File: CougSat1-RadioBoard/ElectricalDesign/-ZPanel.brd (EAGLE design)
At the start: 96 x 96 mm, 50 parts, among them J1 High Gain Antenna, J2 Deployables, J3 High Gain +, J4 ADCS, J5 Flap +X, J6 Flap -X, J7 Flap +Y, J8 Flap -Y, U1 AD7291, U2 AD8542, U3 AD8515

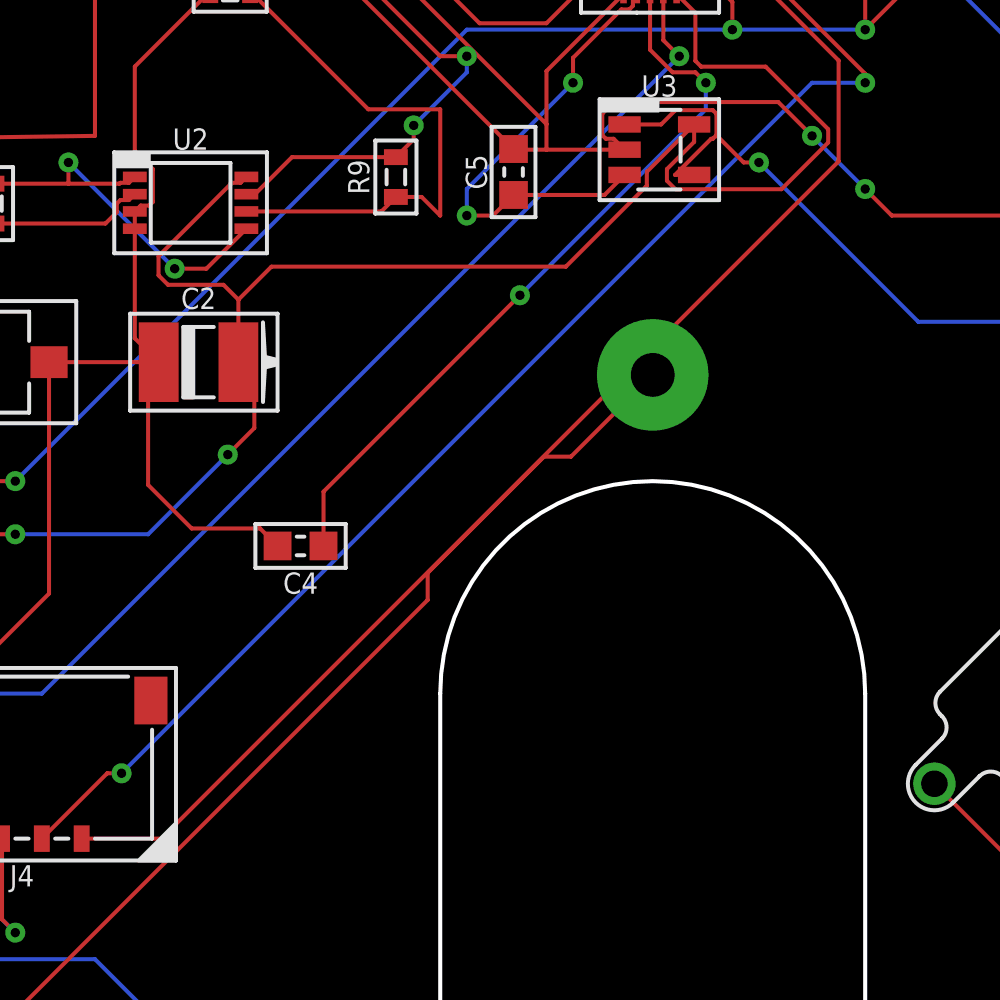
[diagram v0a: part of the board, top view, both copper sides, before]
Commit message: Layout 1.0.0
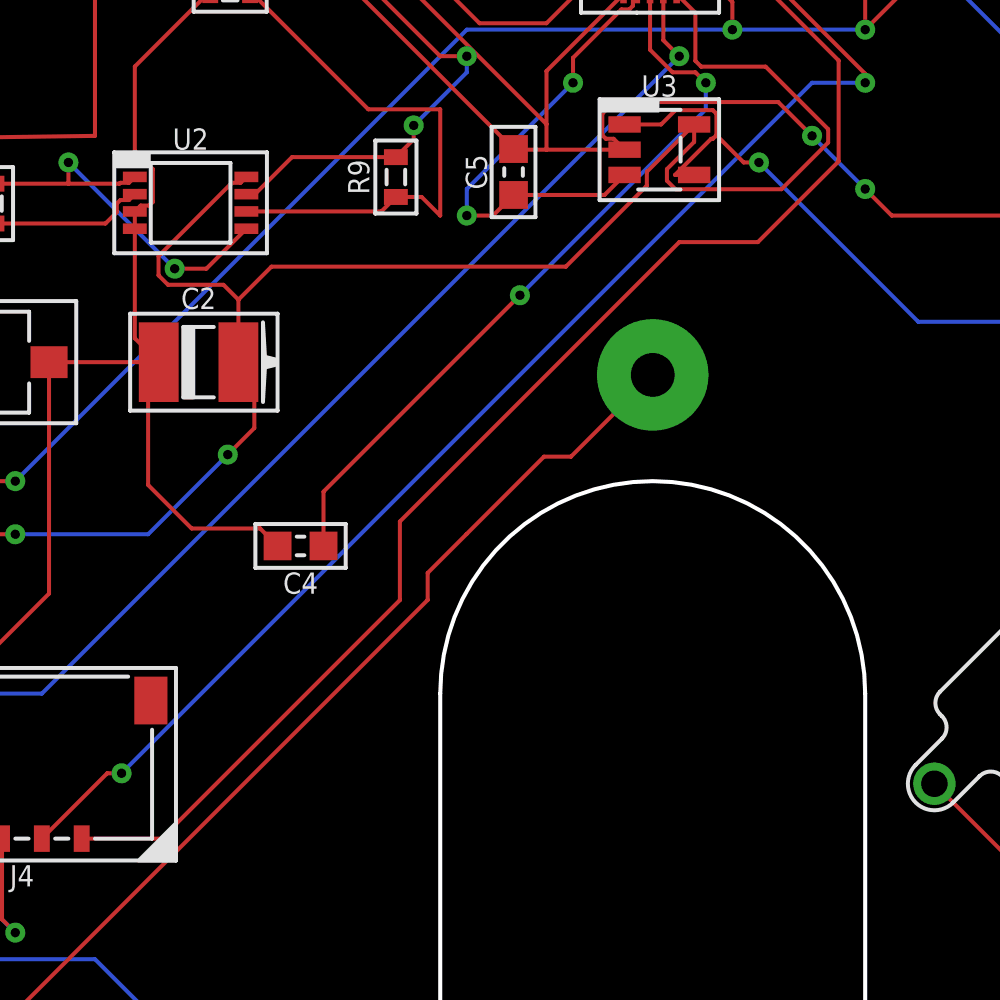
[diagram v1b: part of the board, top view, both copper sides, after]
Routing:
- net I2C_SDA_ADCS: track 50.1 -> 51.8 mm
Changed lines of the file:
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@@
 <contactref element="U1" pad="14"/>
 <contactref element="J4" pad="1"/>
-<wire x1="55" y1="82.04" x2="29.5" y2="56.54" width="0.1524" layer="1"/>
+<wire x1="29.5" y1="56.54" x2="38.48" y2="65.52" width="0.1524" layer="1"/>
 <wire x1="26.5" y1="56.54" x2="29.5" y2="56.54" width="0.1524" layer="1"/>
 <wire x1="50.2446875" y1="90.5936" x2="49.9464" y2="90.5936" width="0.1524" layer="1"/>
@@
 <wire x1="55" y1="85.8382875" x2="50.2446875" y2="90.5936" width="0.1524" layer="1"/>
 <wire x1="55" y1="82.04" x2="55" y2="85.8382875" width="0.1524" layer="1"/>
+<wire x1="38.48" y1="65.52" x2="38.48" y2="68.48" width="0.1524" layer="1"/>
+<wire x1="38.48" y1="68.48" x2="49" y2="79" width="0.1524" layer="1"/>
+<wire x1="49" y1="79" x2="51.96" y2="79" width="0.1524" layer="1"/>
+<wire x1="51.96" y1="79" x2="55" y2="82.04" width="0.1524" layer="1"/>
 </signal>
 <signal name="I2C_SCL_ADCS">
@@
 <wire x1="44.922309375" y1="70.922309375" x2="48" y2="74" width="0.1524" layer="1"/>
 <wire x1="39.526871875" y1="65.526871875" x2="39.526871875" y2="66.542471875" width="0.1524" layer="1"/>
-<wire x1="39.526871875" y1="66.542471875" x2="43.906709375" y2="70.922309375" width="0.1524" layer="1"/>
+<wire x1="39.526871875" y1="66.542471875" x2="40.9922" y2="68.0078" width="0.1524" layer="1"/>
+<wire x1="40.9922" y1="68.0078" x2="43.906709375" y2="70.922309375" width="0.1524" layer="1"/>
 <wire x1="43.906709375" y1="70.922309375" x2="44.922309375" y2="70.922309375" width="0.1524" layer="1"/>
 <wire x1="73.74" y1="47.48" x2="62.25" y2="28" width="0.1524" layer="1"/>
